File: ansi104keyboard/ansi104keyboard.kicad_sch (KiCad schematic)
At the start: 2 parts, among them SW1 SW_Push_45deg

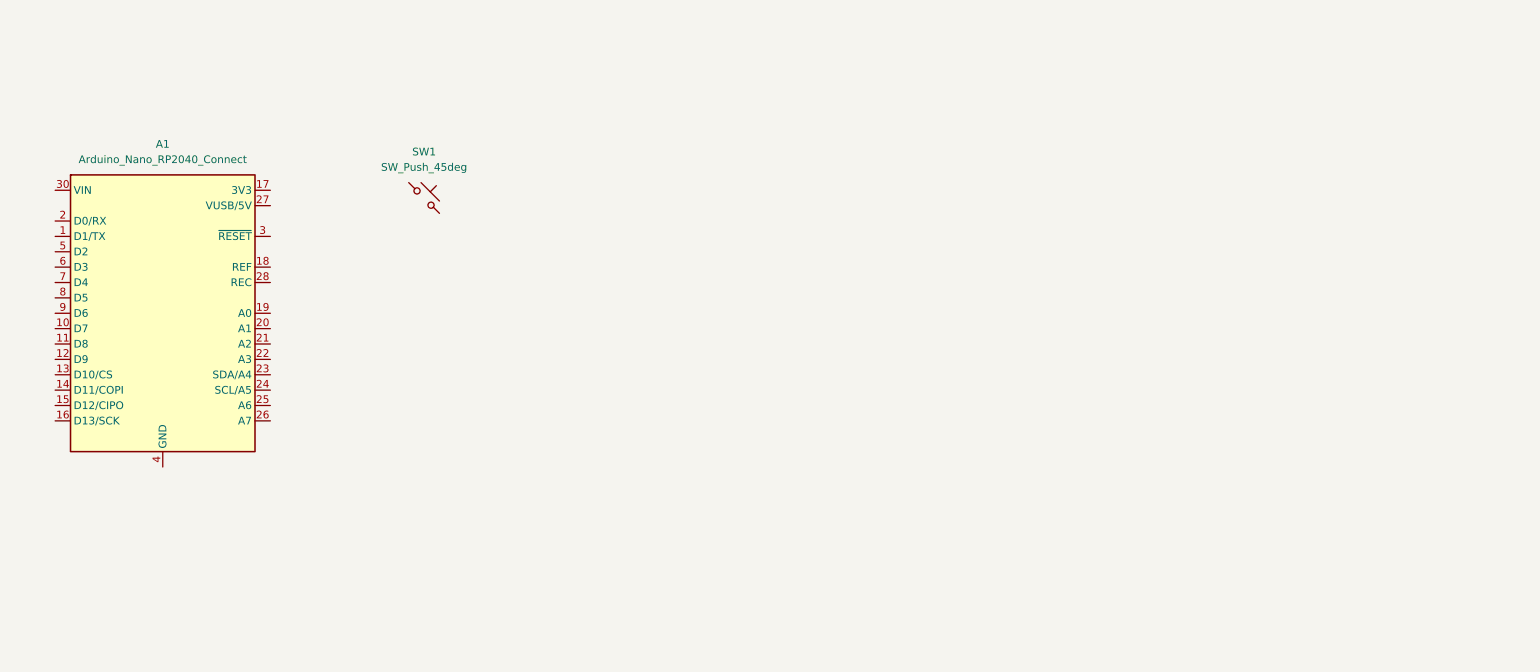
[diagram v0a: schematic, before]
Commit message: updated pcb
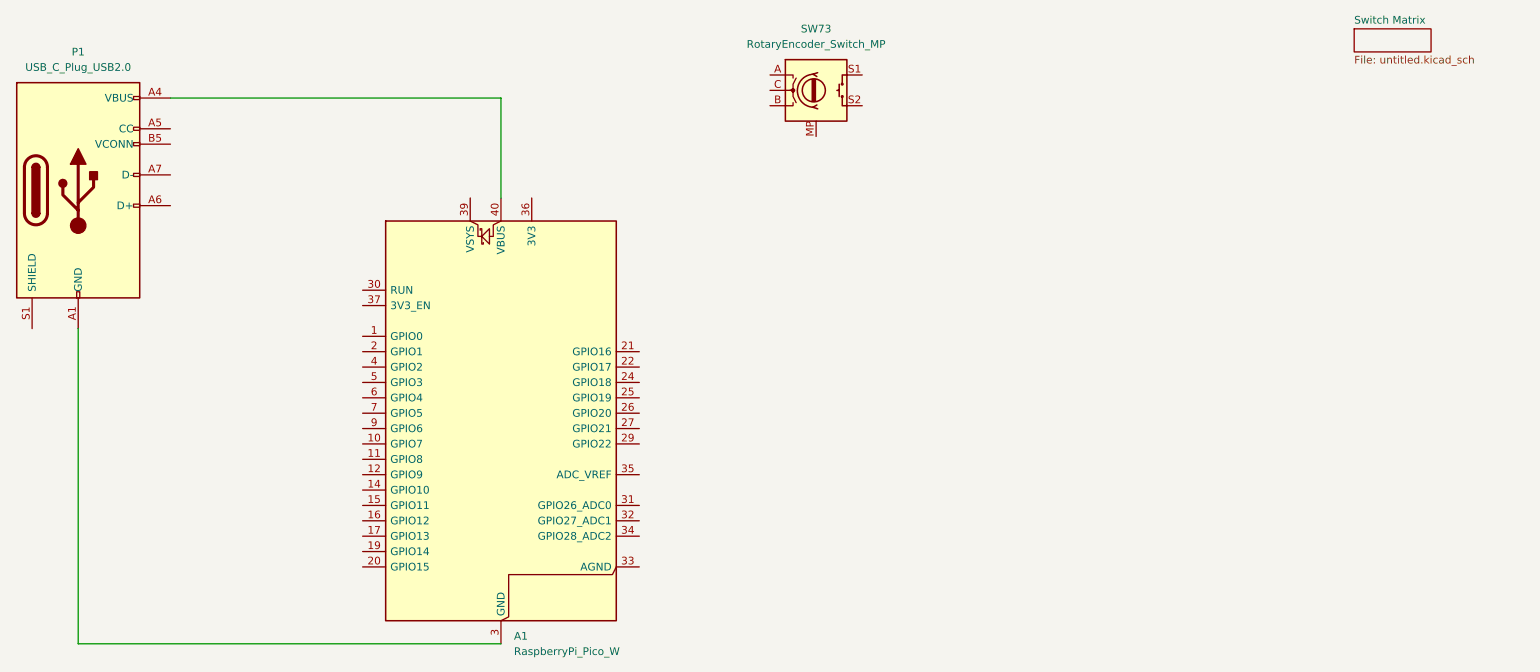
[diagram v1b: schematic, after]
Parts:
- removed A1: Arduino_Nano_RP2040_Connect, Module:Arduino_Nano, symbol MCU_Module:Arduino_Nano_RP2040_Connect
- removed SW1: SW_Push_45deg, symbol Switch:SW_Push_45deg
- added A1: RaspberryPi_Pico_W, Module:RaspberryPi_Pico_W_SMD_HandSolder, symbol MCU_Module:RaspberryPi_Pico_W
- added P1: USB_C_Plug_USB2.0, symbol Connector:USB_C_Plug_USB2.0
- added SW73: RotaryEncoder_Switch_MP, symbol Device:RotaryEncoder_Switch_MP
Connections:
- new net: A1.13 (GND), A1.18 (GND), A1.23 (GND), A1.28 (GND), A1.3 (GND), A1.38 (GND), A1.8 (GND), P1.A1 (GND), P1.A12 (GND), P1.B1 (GND), P1.B12 (GND)
- new net: A1.40 (VBUS), P1.A4 (VBUS), P1.A9 (VBUS), P1.B4 (VBUS), P1.B9 (VBUS)
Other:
- added sheet Switch Matrix (untitled.kicad_sch)
